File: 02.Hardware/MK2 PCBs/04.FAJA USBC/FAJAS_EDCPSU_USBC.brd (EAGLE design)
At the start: 42.8 x 41.6 mm, 28 parts, among them K1 FLEX_DCDC, K2 FLEX_DCDC, K3 FLEX_CONN, K4 FLEX8, K5 FLEX8

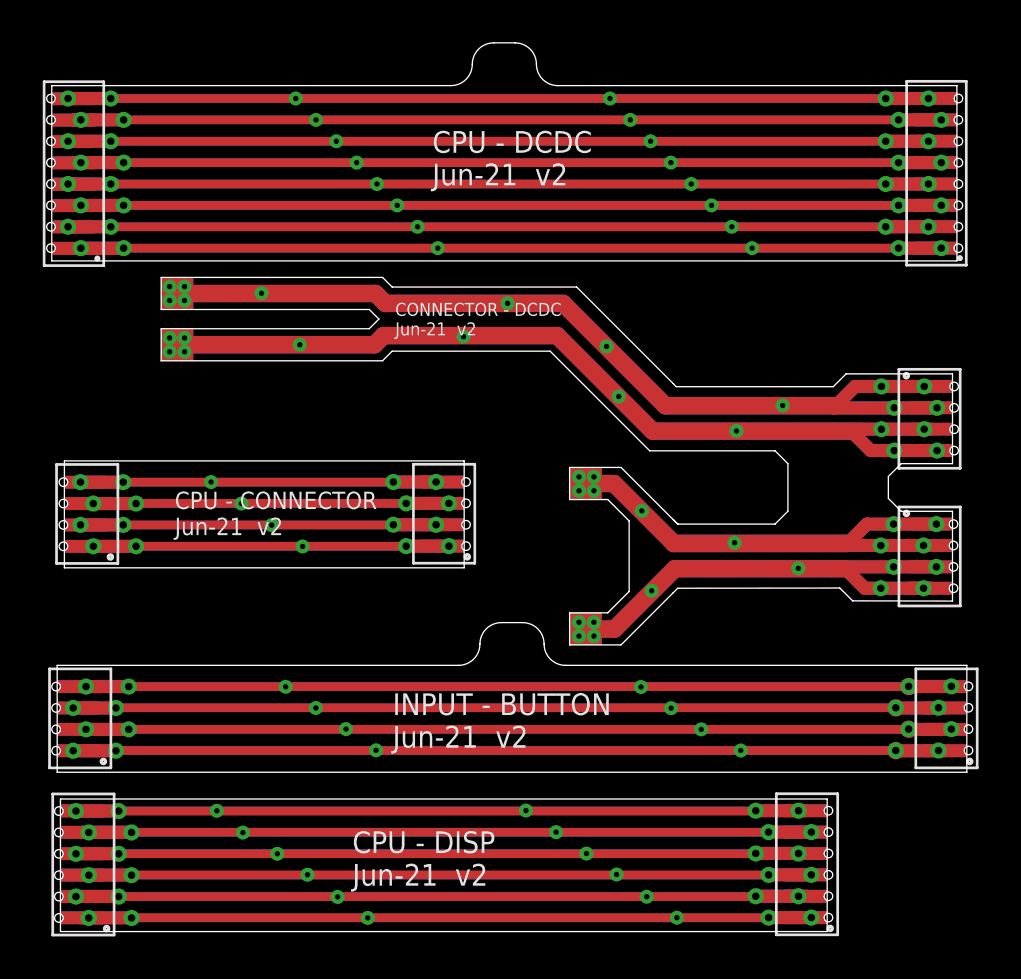
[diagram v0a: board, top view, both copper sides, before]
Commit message: Flex MK2 Creation
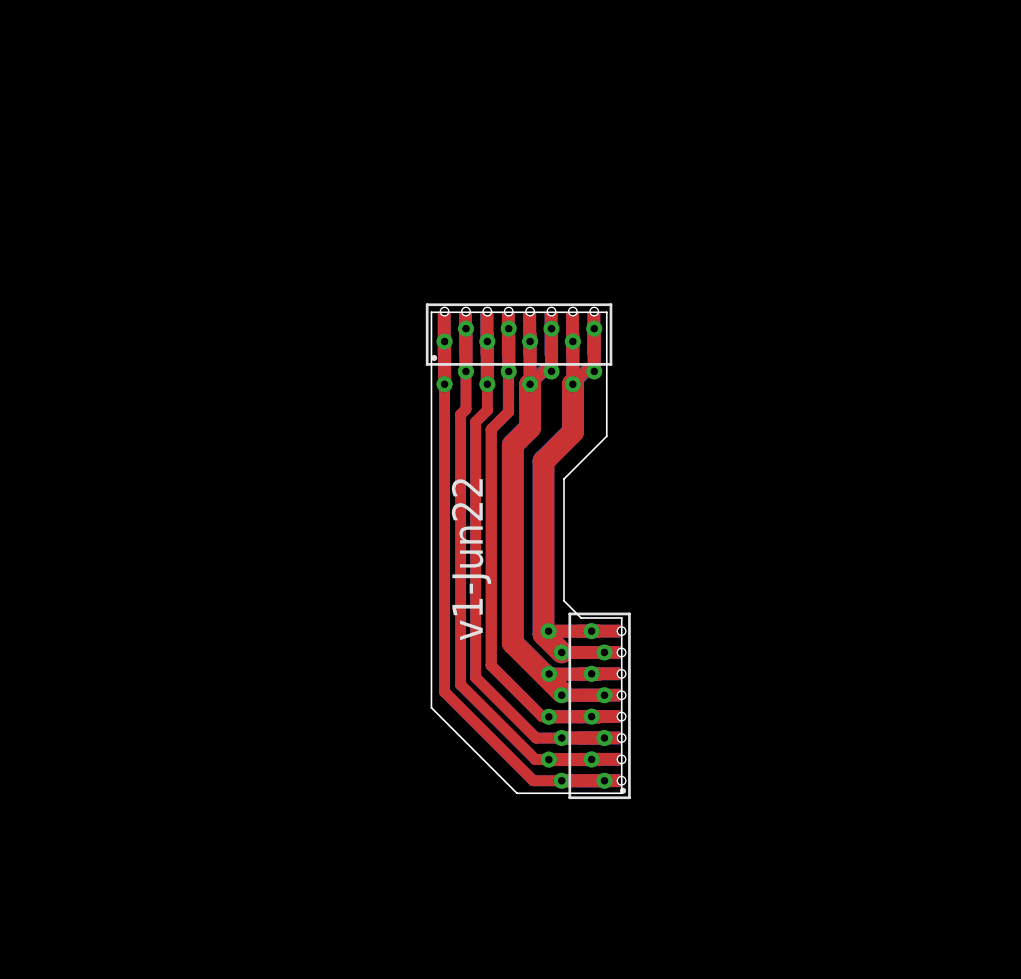
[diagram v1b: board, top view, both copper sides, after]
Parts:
- removed DISP_CPU_1, DISP_CPU_4: DISP_CPU_1, Flex_Faja_connector:FLEX6
- removed DISP_CPU_2, DISP_CPU_3: DISP_CPU_2, Flex_Faja_connector:FLEX6
- removed FLX1, FLX10, FLX11, FLX2, FLX3, FLX4, FLX5, FLX6, FLX7, FLX8, FLX9: FLEX4, Flex4:FLEX4
- removed GND1, GND2, VO+, VO+1, VO-, VO-1, VSYS_IP, VSYS_IP1: TESTPAD_TPSQTP15SQ, BeagleBone_Blue_R3:TESTPAD_TP15SQ
- removed K3: FLEX_CONN, Flex4:FLEX4
- K1, K2: value FLEX_DCDC -> FLEX_MK2
- K4, K5: value FLEX8 -> FLEX_MK2
- moved K4 29.5 mm to (38.6, 24.1)
- moved K5 29.5 mm to (38.1, 24.1)
- moved K1 22.3 mm to (34.6, 41.7), turned to 180 degrees
- moved K2 22.0 mm to (34.6, 41.2), turned to 0 degrees
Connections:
- net CPU-DCDC_1 renamed P-
- net CPU-DCDC_2 renamed P+
- net CPU-DCDC_3 renamed SEL
- net CPU-DCDC_4 renamed VCC
- removed net BUTTON-INPUT_1: FLX1.1, FLX6.1, FLX8.1, FLX9.1
- removed net BUTTON-INPUT_2: FLX1.2, FLX6.2, FLX8.2, FLX9.2
- removed net BUTTON-INPUT_3: FLX1.3, FLX6.3, FLX8.3, FLX9.3
- removed net BUTTON-INPUT_4: FLX1.4, FLX6.4, FLX8.4, FLX9.4
- removed net CPU-CONN_1: FLX10.1, FLX11.1, FLX3.1, K3.1
- removed net CPU-CONN_2: FLX10.2, FLX11.2, FLX3.2, K3.2
- removed net CPU-CONN_3: FLX10.3, FLX11.3, FLX3.3, K3.3
- removed net CPU-CONN_4: FLX10.4, FLX11.4, FLX3.4, K3.4
- removed net CPU-DCDC_5: K1.5, K2.5, K4.5, K5.5
- removed net CPU-DCDC_6: K1.6, K2.6, K4.6, K5.6
- removed net CPU-DCDC_7: K1.7, K2.7, K4.7, K5.7
- removed net CPU-DCDC_8: K1.8, K2.8, K4.8, K5.8
- removed net DSP-CPU_1: DISP_CPU_1.1, DISP_CPU_2.1, DISP_CPU_3.1, DISP_CPU_4.1
- removed net DSP-CPU_2: DISP_CPU_1.2, DISP_CPU_2.2, DISP_CPU_3.2, DISP_CPU_4.2
- removed net DSP-CPU_3: DISP_CPU_1.3, DISP_CPU_2.3, DISP_CPU_3.3, DISP_CPU_4.3
- removed net DSP-CPU_4: DISP_CPU_1.4, DISP_CPU_2.4, DISP_CPU_3.4, DISP_CPU_4.4
- removed net DSP-CPU_5: DISP_CPU_1.5, DISP_CPU_2.5, DISP_CPU_3.5, DISP_CPU_4.5
- removed net DSP-CPU_6: DISP_CPU_1.6, DISP_CPU_2.6, DISP_CPU_3.6, DISP_CPU_4.6
- removed net VOUT+: FLX2.1, FLX2.2, FLX4.1, FLX4.2, VO+.TP, VO+1.TP
- removed net VOUT-: FLX2.3, FLX2.4, FLX4.3, FLX4.4, VO-.TP, VO-1.TP
- removed net VSYS: FLX5.3, FLX5.4, FLX7.3, FLX7.4, VSYS_IP.TP, VSYS_IP1.TP
- new net VOUT: K1.5, K1.6, K2.5, K2.6, K4.5, K4.6, K5.5, K5.6
- net GND: now also K1.7, K1.8, K2.7, K2.8, K4.7, K4.8, K5.7, K5.8; no longer FLX5.1, FLX5.2, FLX7.1, FLX7.2, GND1.TP, GND2.TP
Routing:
- net VOUT+: track 84.8 -> 0.00 mm, vias 10 -> 0
- net VOUT-: track 84.7 -> 0.00 mm, vias 10 -> 0
- net CPU-DCDC_5: track 82.6 -> 0.00 mm, vias 6 -> 0
- net BUTTON-INPUT_4: track 81.4 -> 0.00 mm, vias 6 -> 0
- net BUTTON-INPUT_2: track 81.1 -> 0.00 mm, vias 6 -> 0
- net BUTTON-INPUT_3: track 81.1 -> 0.00 mm, vias 6 -> 0
- net BUTTON-INPUT_1: track 81.1 -> 0.00 mm, vias 6 -> 0
- net CPU-DCDC_7: track 80.7 -> 0.00 mm, vias 6 -> 0
- net CPU-DCDC_6: track 80.7 -> 0.00 mm, vias 6 -> 0
- net CPU-DCDC_8: track 80.3 -> 0.00 mm, vias 6 -> 0
- net DSP-CPU_4: track 70.0 -> 0.00 mm, vias 6 -> 0
- net DSP-CPU_6: track 69.4 -> 0.00 mm, vias 6 -> 0
- net DSP-CPU_2: track 69.4 -> 0.00 mm, vias 6 -> 0
- net DSP-CPU_5: track 68.3 -> 0.00 mm, vias 6 -> 0
- net DSP-CPU_3: track 68.0 -> 0.00 mm, vias 6 -> 0
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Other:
- board size 42.8 x 41.6 mm -> 8.9 x 22.5 mm
- board text added: "v1-Jun22"
- board text removed: "CONNECTOR - DCDC Jun-21 v2"
- board text removed: "CPU - CONNECTOR Jun-21 v2"
- board text removed: "CPU - DCDC Jun-21 v2"
- board text removed: "CPU - DISP Jun-21 v2"
- board text removed: "INPUT - BUTTON Jun-21 v2"
